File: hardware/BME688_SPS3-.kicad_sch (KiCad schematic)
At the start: 15 parts, among them U401 TPS613222ADBVR, U402 BME688, U403 USBLC6-2P6

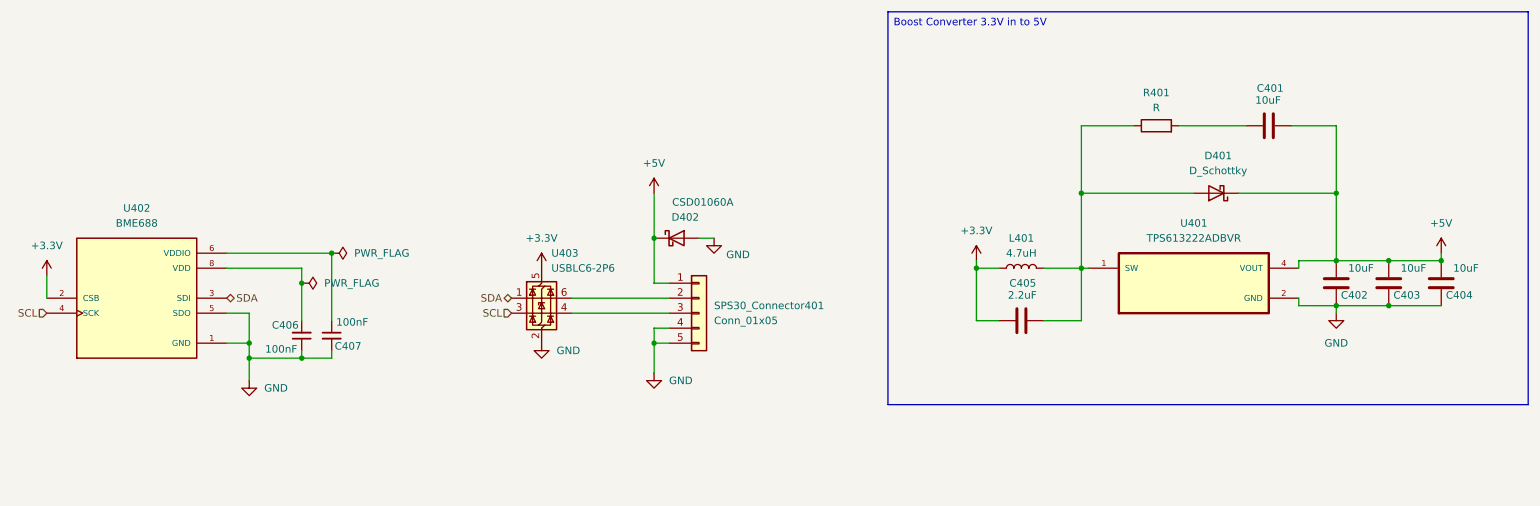
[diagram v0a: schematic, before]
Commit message: power layout WIP
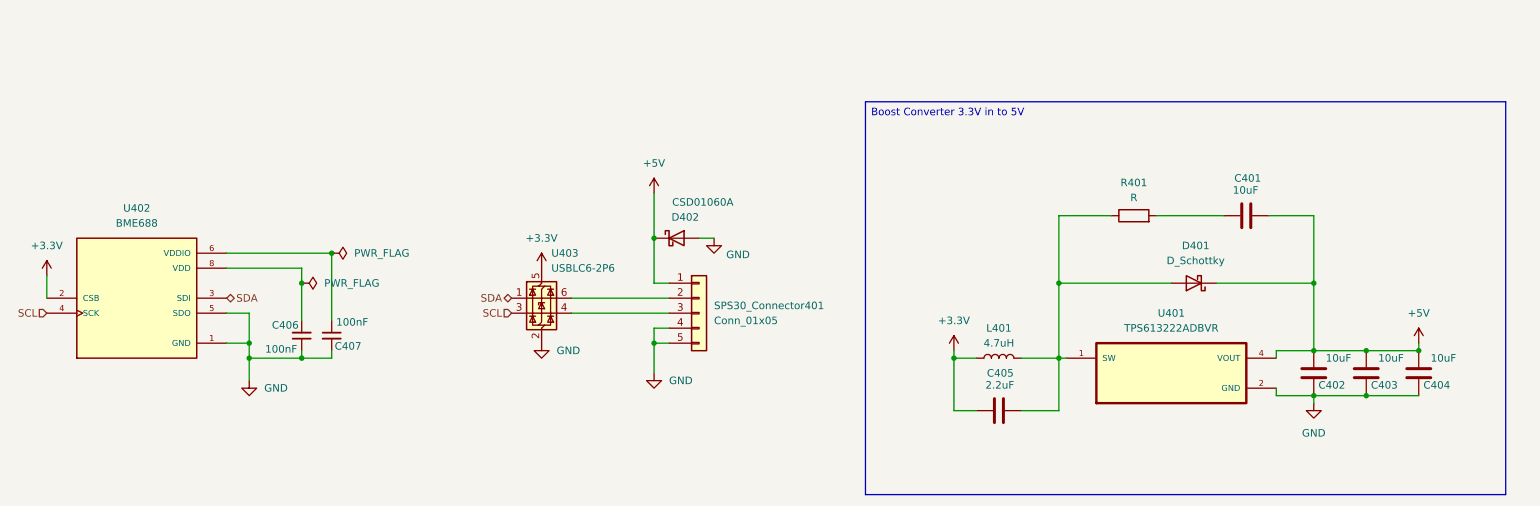
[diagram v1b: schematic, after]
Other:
- moved on the sheet: C401, C402, C403, C404, C405, D401, L401, R401, U401

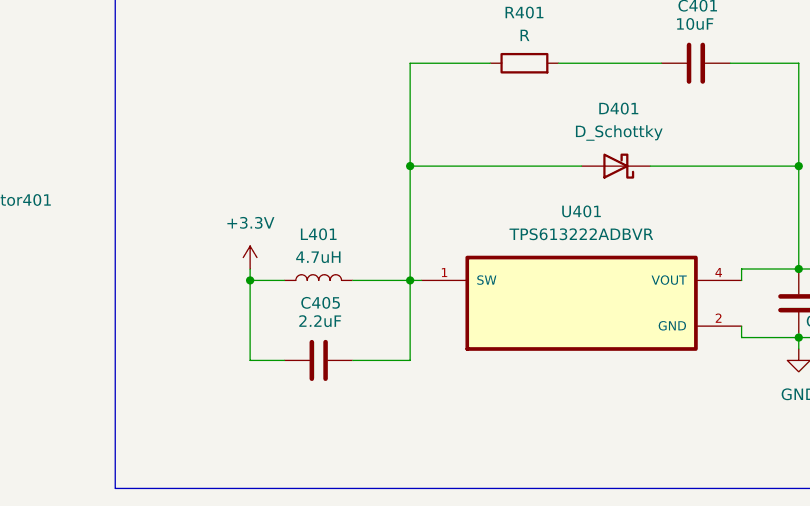
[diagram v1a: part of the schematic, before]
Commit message: PCB update
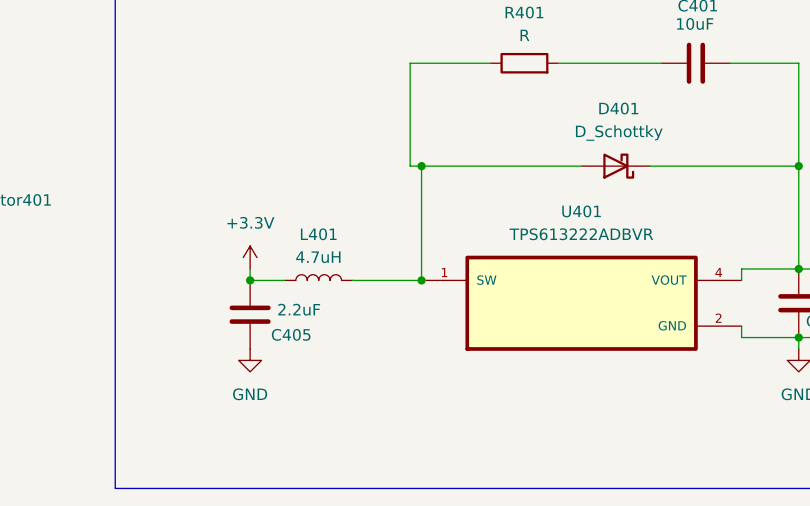
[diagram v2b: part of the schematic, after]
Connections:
- net GND: now also C405.1
- net at D401.2 (A), L401.2, R401.1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: no longer C405.1
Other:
- moved on the sheet: C405
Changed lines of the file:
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@@
+	)
+	(junction
+		(at 201.93 119.38)
+		(diameter 0)
+		(color 0 0 0 0)
 	)
 	(junction
@@
 	)
 	(junction
-		(at 132.08 99.06)
+		(at 201.93 106.68)
 		(diameter 0)
 		(color 0 0 0 0)
 	)
 	(junction
-		(at 200.66 119.38)
+		(at 132.08 99.06)
 		(diameter 0)
 		(color 0 0 0 0)
@@
 	)
 	(junction
-		(at 200.66 106.68)
+		(at 252.73 118.11)
+		(diameter 0)
+		(color 0 0 0 0)
+	)
+	(junction
+		(at 243.84 106.68)
 		(diameter 0)
 		(color 0 0 0 0)
@@
 		(color 0 0 0 0)
 	)
-	(junction
-		(at 252.73 118.11)
-		(diameter 0)
-		(color 0 0 0 0)
-	)
-	(junction
-		(at 243.84 106.68)
-		(diameter 0)
-		(color 0 0 0 0)
-	)
 	(wire
 		(pts
@@
 	(wire
 		(pts
-			(xy 194.31 119.38) (xy 200.66 119.38)
-		)
-		(stroke
-			(width 0)
-			(type default)
-		)
-	)
-	(wire
-		(pts
 			(xy 77.47 118.11) (xy 77.47 119.38)
 		)
@@
 	(wire
 		(pts
-			(xy 200.66 119.38) (xy 200.66 128.27)
-		)
-		(stroke
-			(width 0)
-			(type default)
-		)
-	)
-	(wire
-		(pts
 			(xy 243.84 106.68) (xy 243.84 118.11)
 		)
@@
 	(wire
 		(pts
-			(xy 182.88 119.38) (xy 182.88 128.27)
-		)
-		(stroke
-			(width 0)
-			(type default)
-		)
-	)
-	(wire
-		(pts
 			(xy 243.84 125.73) (xy 252.73 125.73)
 		)
@@
 	(wire
 		(pts
+			(xy 201.93 106.68) (xy 219.71 106.68)
+		)
+		(stroke
+			(width 0)
+			(type default)
+		)
+	)
+	(wire
+		(pts
 			(xy 29.21 105.41) (xy 29.21 109.22)
 		)
@@
 	(wire
 		(pts
+			(xy 201.93 106.68) (xy 200.66 106.68)
+		)
+		(stroke
+			(width 0)
+			(type default)
+		)
+	)
+	(wire
+		(pts
 			(xy 132.08 116.84) (xy 134.62 116.84)
 		)
@@
 	(wire
 		(pts
-			(xy 182.88 128.27) (xy 186.69 128.27)
-		)
-		(stroke
-			(width 0)
-			(type default)
-		)
-	)
-	(wire
-		(pts
 			(xy 59.69 101.6) (xy 77.47 101.6)
 		)
@@
 	(wire
 		(pts
-			(xy 194.31 128.27) (xy 200.66 128.27)
-		)
-		(stroke
-			(width 0)
-			(type default)
-		)
-	)
-	(wire
-		(pts
 			(xy 132.08 99.06) (xy 132.08 106.68)
 		)
@@
 	(wire
 		(pts
-			(xy 200.66 119.38) (xy 201.93 119.38)
-		)
-		(stroke
-			(width 0)
-			(type default)
-		)
-	)
-	(wire
-		(pts
 			(xy 72.39 118.11) (xy 72.39 119.38)
 		)
@@
 	(wire
 		(pts
-			(xy 200.66 119.38) (xy 200.66 106.68)
-		)
-		(stroke
-			(width 0)
-			(type default)
-		)
-	)
-	(wire
-		(pts
-			(xy 200.66 106.68) (xy 219.71 106.68)
+			(xy 201.93 119.38) (xy 201.93 106.68)
+		)
+		(stroke
+			(width 0)
+			(type default)
+		)
+	)
+	(wire
+		(pts
+			(xy 194.31 119.38) (xy 201.93 119.38)
 		)
 		(stroke
@@
 	(symbol
 		(lib_id "Device:C")
-		(at 190.5 128.27 270)
+		(at 182.88 123.19 180)
 		(unit 1)
 		(exclude_from_sim no)
@@
 		(dnp no)
 		(property "Reference" "C405"
-			(at 188.468 121.92 90)
+			(at 189.738 125.476 0)
 			(effects
 				(font
@@
 		)
 		(property "Value" "2.2uF"
-			(at 188.214 123.952 90)
+			(at 190.754 122.682 0)
 			(effects
 				(font
@@
 		)
 		(property "Footprint" "Capacitor_SMD:C_0603_1608Metric"
-			(at 186.69 129.2352 0)
+			(at 181.9148 119.38 0)
 			(effects
 				(font
@@
 		)
 		(property "Datasheet" "~"
-			(at 190.5 128.27 0)
+			(at 182.88 123.19 0)
 			(effects
 				(font
@@
 		)
 		(property "Description" "Unpolarized capacitor"
-			(at 190.5 128.27 0)
+			(at 182.88 123.19 0)
 			(effects
 				(font
@@
 					(unit 1)
 				)
+			)
+		)
+	)
+	(symbol
+		(lib_id "power:GND")
+		(at 182.88 127 0)
+		(unit 1)
+		(exclude_from_sim no)
+		(in_bom yes)
+		(on_board yes)
+		(dnp no)
+		(fields_autoplaced yes)
+		(property "Reference" "#PWR0411"
+			(at 182.88 133.35 0)
+			(effects
+				(font
+					(size 1.27 1.27)
+				)
+				(hide yes)
+			)
+		)
+		(property "Value" "GND"
+			(at 182.88 132.08 0)
+			(effects
+				(font
+					(size 1.27 1.27)
+				)
+			)
+		)
+		(property "Footprint" ""
+			(at 182.88 127 0)
+			(effects
+				(font
+					(size 1.27 1.27)
+				)
+				(hide yes)
+			)
+		)
+		(property "Datasheet" ""
+			(at 182.88 127 0)
+			(effects
+				(font
+					(size 1.27 1.27)
+				)
+				(hide yes)
+			)
+		)
+		(property "Description" "Power symbol creates a global label with name \"GND\" , ground"
+			(at 182.88 127 0)
+			(effects
+				(font
+					(size 1.27 1.27)
+				)
+				(hide yes)
+			)
+		)
+		(pin "1"
+		)
+		(instances
+			(project "Senior_Design"
+				(path "/8f5928e8-0fc1-4443-a20f-3bfeb956761e/140ad835-eaa4-4a8c-a4e7-0525bbf22a2e"
+					(reference "#PWR0411")
+					(unit 1)
+				)
